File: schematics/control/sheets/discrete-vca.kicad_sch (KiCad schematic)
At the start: 18 parts, among them Q2 2N3904, Q3 2N3904, U10 TL072

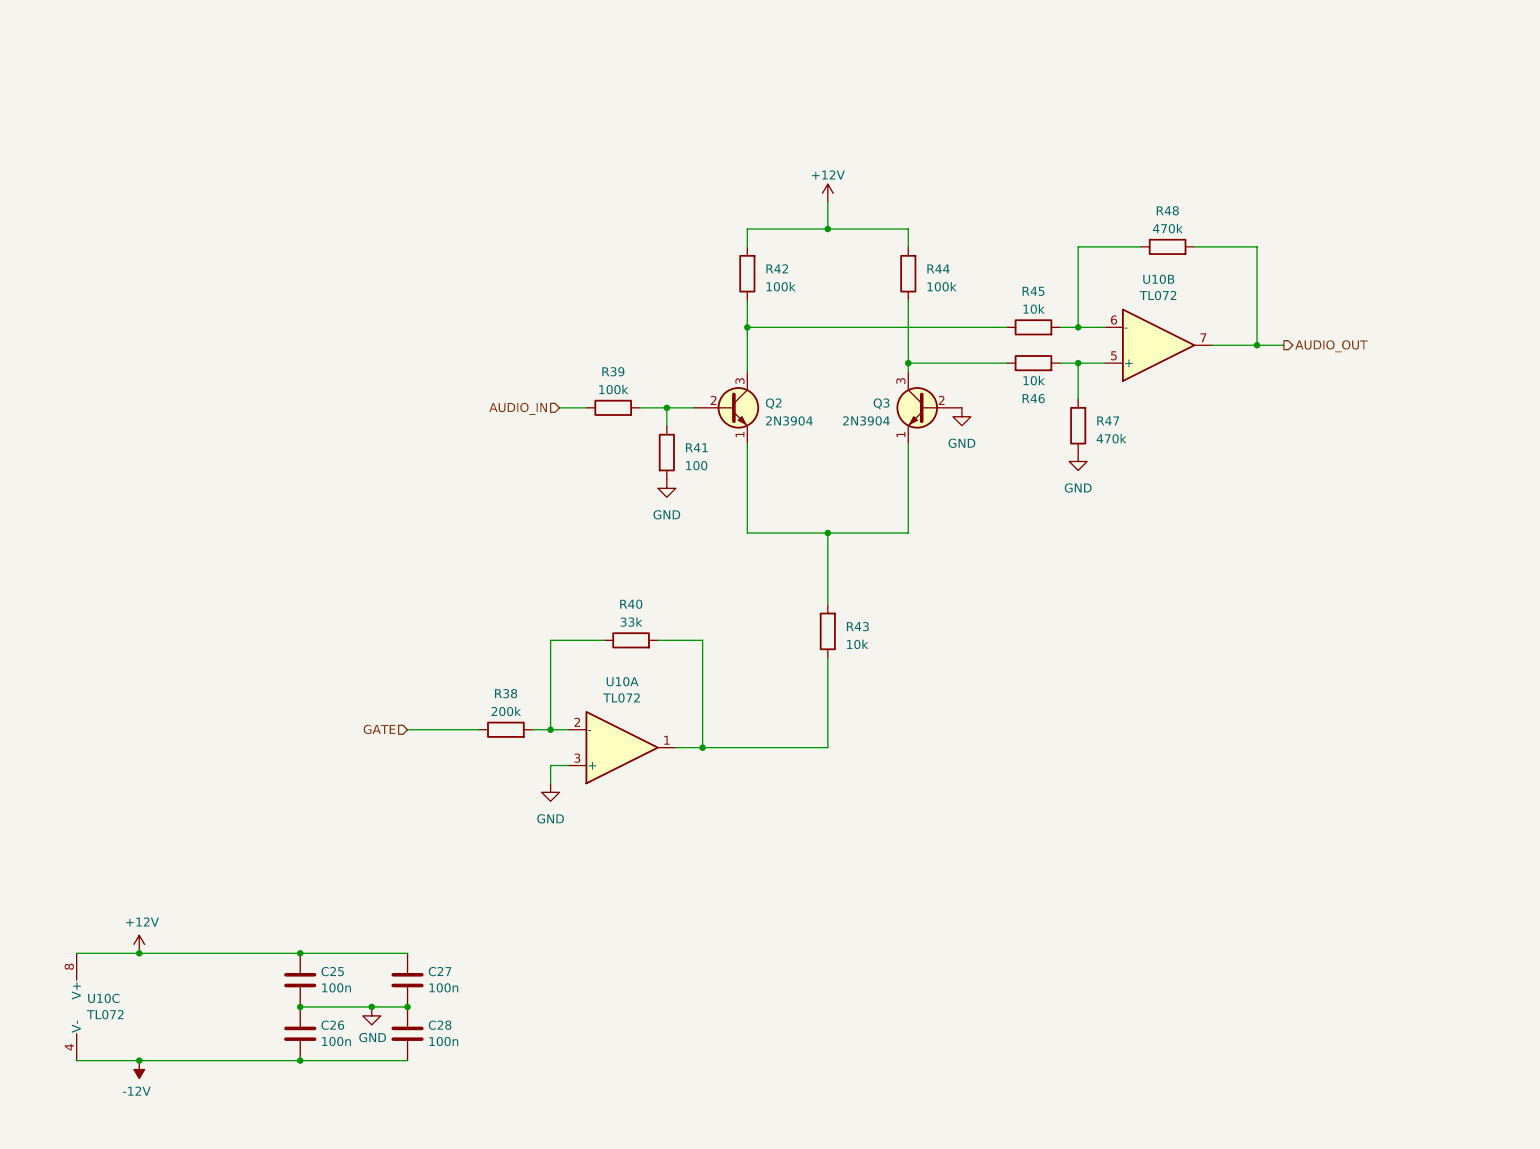
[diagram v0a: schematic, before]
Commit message: Updated VCA
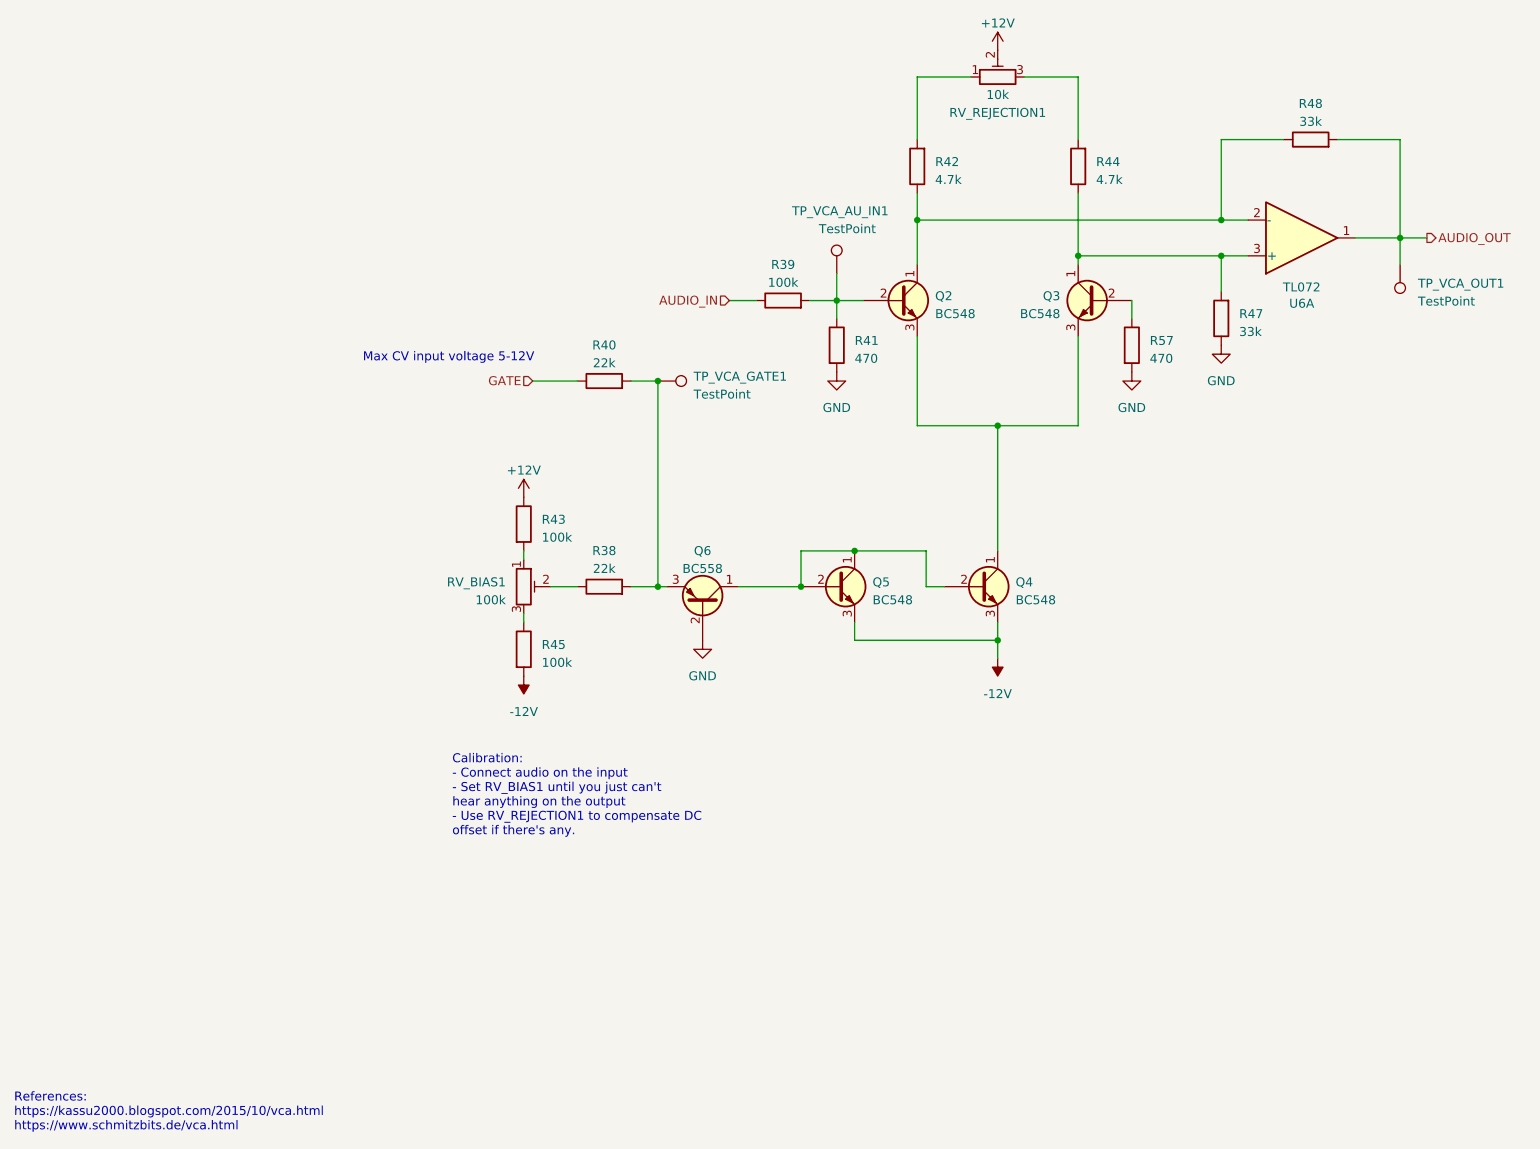
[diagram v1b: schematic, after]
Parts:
- removed C25, C26, C27, C28: 100n, Capacitor_THT:C_Disc_D3.0mm_W2.0mm_P2.50mm, symbol Device:C
- removed Q2, Q3: 2N3904, Package_TO_SOT_THT_AKL:TO-92_Inline_Wide_EBC, symbol PCM_Transistor_BJT_AKL:2N3904
- removed R46: 10k, symbol Device:R
- removed U10: TL072, Package_DIP:DIP-8_W7.62mm, symbol Amplifier_Operational:TL072
- added Q2, Q3, Q4, Q5: BC548, Package_TO_SOT_THT_AKL:TO-92_Inline_Wide_CBE, symbol PCM_Transistor_BJT_AKL:BC548
- added Q6: BC558, Package_TO_SOT_THT_AKL:TO-92_Inline_Wide_CBE, symbol PCM_Transistor_BJT_AKL:BC558
- added R57: 470, symbol Device:R
- added RV_BIAS1: 100k, symbol Device:R_Potentiometer_Trim
- added RV_REJECTION1: 10k, symbol Device:R_Potentiometer_Trim
- added TP_VCA_AU_IN1, TP_VCA_GATE1, TP_VCA_OUT1: TestPoint, symbol Connector:TestPoint
- added U6: TL072, Package_DIP:DIP-8_W7.62mm, symbol Amplifier_Operational:TL072
- R38: value 200k -> 22k
- R40: value 33k -> 22k
- R41: value 100 -> 470
- R42, R44: value 100k -> 4.7k
- R43, R45: value 10k -> 100k
- R47, R48: value 470k -> 33k
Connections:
- net +12V: now also R43.1, RV_REJECTION1.2; no longer R42.2, R44.2
- net -12V: now also R45.2, Q4.3 (E), Q5.3 (E)
- net AUDIO_OUT: now also TP_VCA_OUT1.1, U6.1
- net GATE: now also R40.1; no longer R38.1
- net GND: now also Q6.2 (B), R57.2
- net at R40.2: now also R38.2, Q6.3 (E), TP_VCA_GATE1.1; no longer R43.1
- net at R43.2: now also RV_BIAS1.1
- net at R47.2: now also R44.1, Q3.1 (C), U6.3 (+)
- net at R39.2, R41.1: now also Q2.2 (B), TP_VCA_AU_IN1.1
- net at R42.1: now also R48.1, Q2.1 (C), U6.2 (-); no longer R45.1
- new net: Q2.3 (E), Q3.3 (E), Q4.1 (C)
- new net: R42.2, RV_REJECTION1.1
- new net: R44.2, RV_REJECTION1.3
- new net: R38.1, RV_BIAS1.2
- new net: R45.1, RV_BIAS1.3
- new net: Q4.2 (B), Q5.1 (C), Q5.2 (B), Q6.1 (C)
- new net: Q3.2 (B), R57.1
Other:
- note added: "Calibration: - Connect audio on the input - Set RV_BIAS1 until you just can't hear anything on the output - Use RV_REJECTION1 to compensate DC offset if there's any."
- note added: "Max CV input voltage 5-12V"
- note added: "References: https://kassu2000.blogspot.com/2015/10/vca.html https://www.schmitzbits.de/vca.html"
- company: (none) -> Shmøergh
- title: (none) -> Discrete linear VCA
- moved on the sheet: R39, R41, R42, R44, R47, R48
